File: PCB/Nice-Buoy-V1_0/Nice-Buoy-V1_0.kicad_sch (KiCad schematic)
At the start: 4 parts

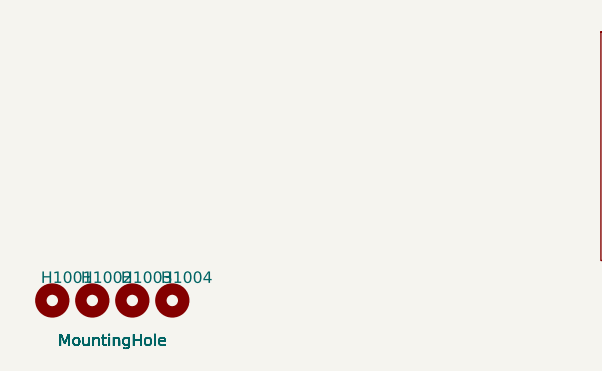
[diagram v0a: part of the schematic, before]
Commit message: PCB finished and orderd at JLCPCB
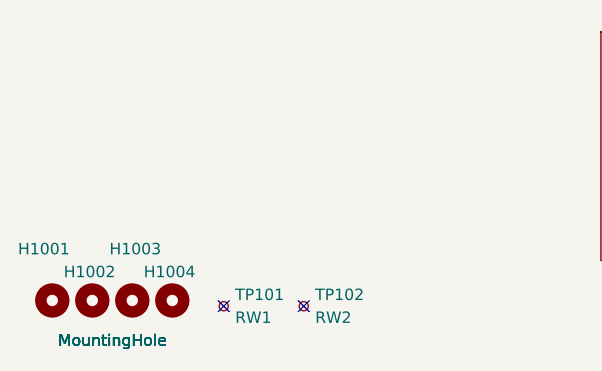
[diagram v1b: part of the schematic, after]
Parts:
- added TP101: RW1, A_Misc:ReworkPins, symbol Connector:TestPoint_Small
- added TP102: RW2, A_Misc:ReworkPins, symbol Connector:TestPoint_Small
- H1001, H1002, H1003, H1004: now left out of the parts list
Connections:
- no-connect marks 0 -> 2
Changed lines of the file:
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@@
   (junction (at 86.36 58.42) (diameter 0) (color 0 0 0 0)
   )
+  (no_connect (at 36.83 191.77))
+  (no_connect (at 45.72 191.77))
   (wire (pts (xy 139.7 105.41) (xy 158.75 105.41))
     (stroke (width 0) (type default))
@@
     (effects (font (size 1.27 1.27)) (justify left bottom))
   )
+  (symbol (lib_id "Connector:TestPoint_Small") (at 45.72 191.77 0) (unit 1)
+    (in_bom no) (on_board yes) (dnp no) (fields_autoplaced)
+    (property "Reference" "TP102" (at 46.99 190.5 0)
+      (effects (font (size 1.27 1.27)) (justify left))
+    )
+    (property "Value" "RW2" (at 46.99 193.04 0)
+      (effects (font (size 1.27 1.27)) (justify left))
+    )
+    (property "Footprint" "A_Misc:ReworkPins" (at 50.8 191.77 0)
+      (effects (font (size 1.27 1.27)) hide)
+    )
+    (property "Datasheet" "~" (at 50.8 191.77 0)
+      (effects (font (size 1.27 1.27)) hide)
+    )
+    (pin "1")
+    (instances
+      (project "Nice-Buoy-V1_0"
+        (path "/77bea089-a6ae-4a6f-b95b-7a9010ad7c5d/20fb3964-c9d0-4636-b697-42bcddc45d6f"
+          (reference "TP102") (unit 1)
+        )
+        (path "/77bea089-a6ae-4a6f-b95b-7a9010ad7c5d"
+          (reference "TP2") (unit 1)
+        )
+      )
+    )
+  )
   (symbol (lib_id "Mechanical:MountingHole") (at 31.115 191.135 0) (unit 1)
-    (in_bom yes) (on_board yes) (dnp no)
-    (property "Reference" "H1004" (at 29.845 188.595 0)
+    (in_bom no) (on_board yes) (dnp no)
+    (property "Reference" "H1004" (at 27.94 187.96 0)
       (effects (font (size 1.27 1.27)) (justify left))
     )
@@
     )
     (instances
-      (project "Nice-Buoy-V1.0"
+      (project "Nice-Buoy-V1_0"
         (path "/77bea089-a6ae-4a6f-b95b-7a9010ad7c5d"
           (reference "H1004") (unit 1)
@@
   )
   (symbol (lib_id "Mechanical:MountingHole") (at 26.67 191.135 0) (unit 1)
-    (in_bom yes) (on_board yes) (dnp no)
-    (property "Reference" "H1003" (at 25.4 188.595 0)
+    (in_bom no) (on_board yes) (dnp no)
+    (property "Reference" "H1003" (at 24.13 185.42 0)
       (effects (font (size 1.27 1.27)) (justify left))
     )
@@
     )
     (instances
-      (project "Nice-Buoy-V1.0"
+      (project "Nice-Buoy-V1_0"
         (path "/77bea089-a6ae-4a6f-b95b-7a9010ad7c5d"
           (reference "H1003") (unit 1)
@@
     )
   )
+  (symbol (lib_id "Connector:TestPoint_Small") (at 36.83 191.77 0) (unit 1)
+    (in_bom no) (on_board yes) (dnp no) (fields_autoplaced)
+    (property "Reference" "TP101" (at 38.1 190.5 0)
+      (effects (font (size 1.27 1.27)) (justify left))
+    )
+    (property "Value" "RW1" (at 38.1 193.04 0)
+      (effects (font (size 1.27 1.27)) (justify left))
+    )
+    (property "Footprint" "A_Misc:ReworkPins" (at 41.91 191.77 0)
+      (effects (font (size 1.27 1.27)) hide)
+    )
+    (property "Datasheet" "~" (at 41.91 191.77 0)
+      (effects (font (size 1.27 1.27)) hide)
+    )
+    (pin "1")
+    (instances
+      (project "Nice-Buoy-V1_0"
+        (path "/77bea089-a6ae-4a6f-b95b-7a9010ad7c5d/20fb3964-c9d0-4636-b697-42bcddc45d6f"
+          (reference "TP101") (unit 1)
+        )
+        (path "/77bea089-a6ae-4a6f-b95b-7a9010ad7c5d"
+          (reference "TP1") (unit 1)
+        )
+      )
+    )
+  )
   (symbol (lib_id "Mechanical:MountingHole") (at 22.225 191.135 0) (unit 1)
-    (in_bom yes) (on_board yes) (dnp no)
-    (property "Reference" "H1002" (at 20.955 188.595 0)
+    (in_bom no) (on_board yes) (dnp no)
+    (property "Reference" "H1002" (at 19.05 187.96 0)
       (effects (font (size 1.27 1.27)) (justify left))
     )
@@
     )
     (instances
-      (project "Nice-Buoy-V1.0"
+      (project "Nice-Buoy-V1_0"
         (path "/77bea089-a6ae-4a6f-b95b-7a9010ad7c5d"
           (reference "H1002") (unit 1)
@@
   )
   (symbol (lib_id "Mechanical:MountingHole") (at 17.78 191.135 0) (unit 1)
-    (in_bom yes) (on_board yes) (dnp no)
-    (property "Reference" "H1001" (at 16.51 188.595 0)
+    (in_bom no) (on_board yes) (dnp no)
+    (property "Reference" "H1001" (at 13.97 185.42 0)
       (effects (font (size 1.27 1.27)) (justify left))
     )
@@
     )
     (instances
-      (project "Nice-Buoy-V1.0"
+      (project "Nice-Buoy-V1_0"
         (path "/77bea089-a6ae-4a6f-b95b-7a9010ad7c5d"
           (reference "H1001") (unit 1)
@@
     )
     (instances
-      (project "Nice-Buoy-V1.0"
+      (project "Nice-Buoy-V1_0"
         (path "/77bea089-a6ae-4a6f-b95b-7a9010ad7c5d" (page "7"))
       )
@@
     )
     (instances
-      (project "Nice-Buoy-V1.0"
+      (project "Nice-Buoy-V1_0"
         (path "/77bea089-a6ae-4a6f-b95b-7a9010ad7c5d" (page "6"))
       )
@@
     )
     (instances
-      (project "Nice-Buoy-V1.0"
+      (project "Nice-Buoy-V1_0"
         (path "/77bea089-a6ae-4a6f-b95b-7a9010ad7c5d" (page "1"))
       )
@@
     )
     (instances
-      (project "Nice-Buoy-V1.0"
+      (project "Nice-Buoy-V1_0"
         (path "/77bea089-a6ae-4a6f-b95b-7a9010ad7c5d" (page "5"))
       )
@@
     )
     (instances
-      (project "Nice-Buoy-V1.0"
+      (project "Nice-Buoy-V1_0"
         (path "/77bea089-a6ae-4a6f-b95b-7a9010ad7c5d" (page "3"))
       )
@@
     )
     (instances
-      (project "Nice-Buoy-V1.0"
+      (project "Nice-Buoy-V1_0"
         (path "/77bea089-a6ae-4a6f-b95b-7a9010ad7c5d" (page "8"))
       )
@@
     )
     (instances
-      (project "Nice-Buoy-V1.0"
+      (project "Nice-Buoy-V1_0"
         (path "/77bea089-a6ae-4a6f-b95b-7a9010ad7c5d" (page "2"))
       )
@@
     )
     (instances
-      (project "Nice-Buoy-V1.0"
+      (project "Nice-Buoy-V1_0"
         (path "/77bea089-a6ae-4a6f-b95b-7a9010ad7c5d" (page "9"))
       )
@@
     )
     (instances
-      (project "Nice-Buoy-V1.0"
+      (project "Nice-Buoy-V1_0"
         (path "/77bea089-a6ae-4a6f-b95b-7a9010ad7c5d" (page "4"))
       )
